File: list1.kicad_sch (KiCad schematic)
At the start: 10 parts, among them U1 8284A, U2 8259A, U22 74LS04, U3 8088, Y1 14.31818MHz

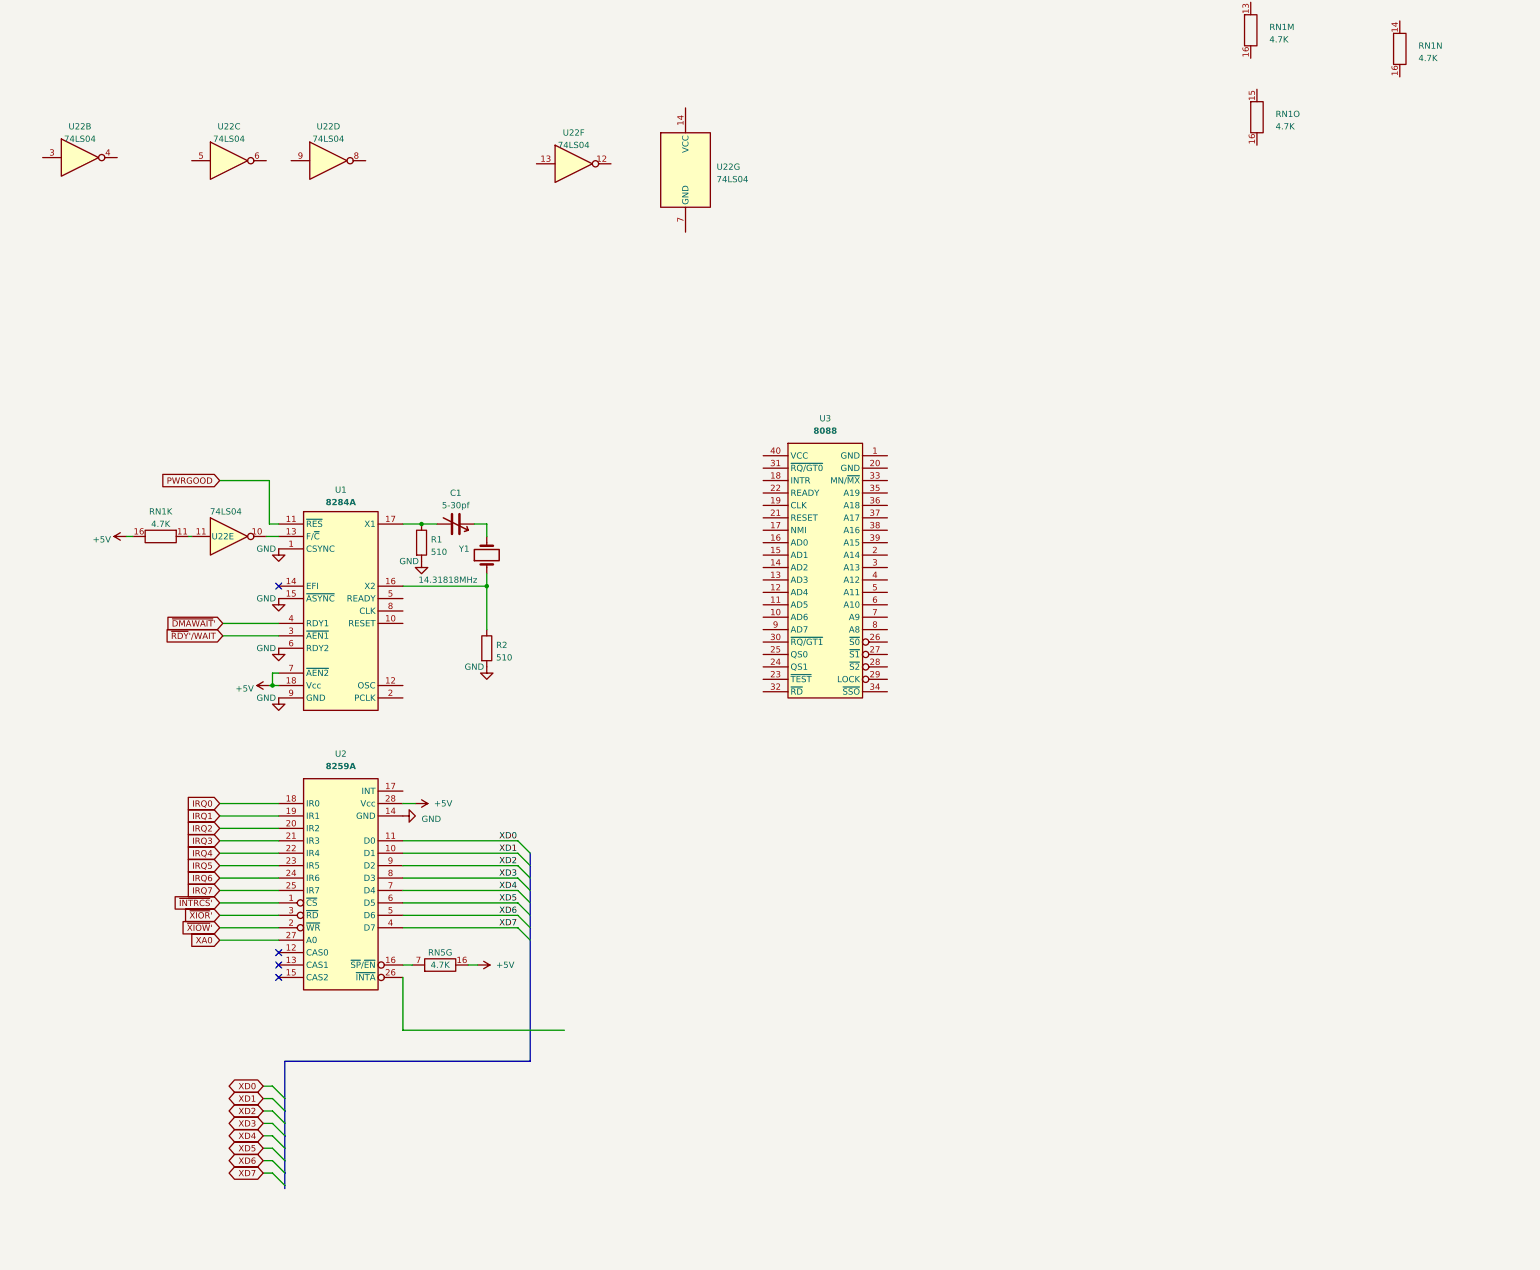
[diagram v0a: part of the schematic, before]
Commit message: Small update 18.04.2024
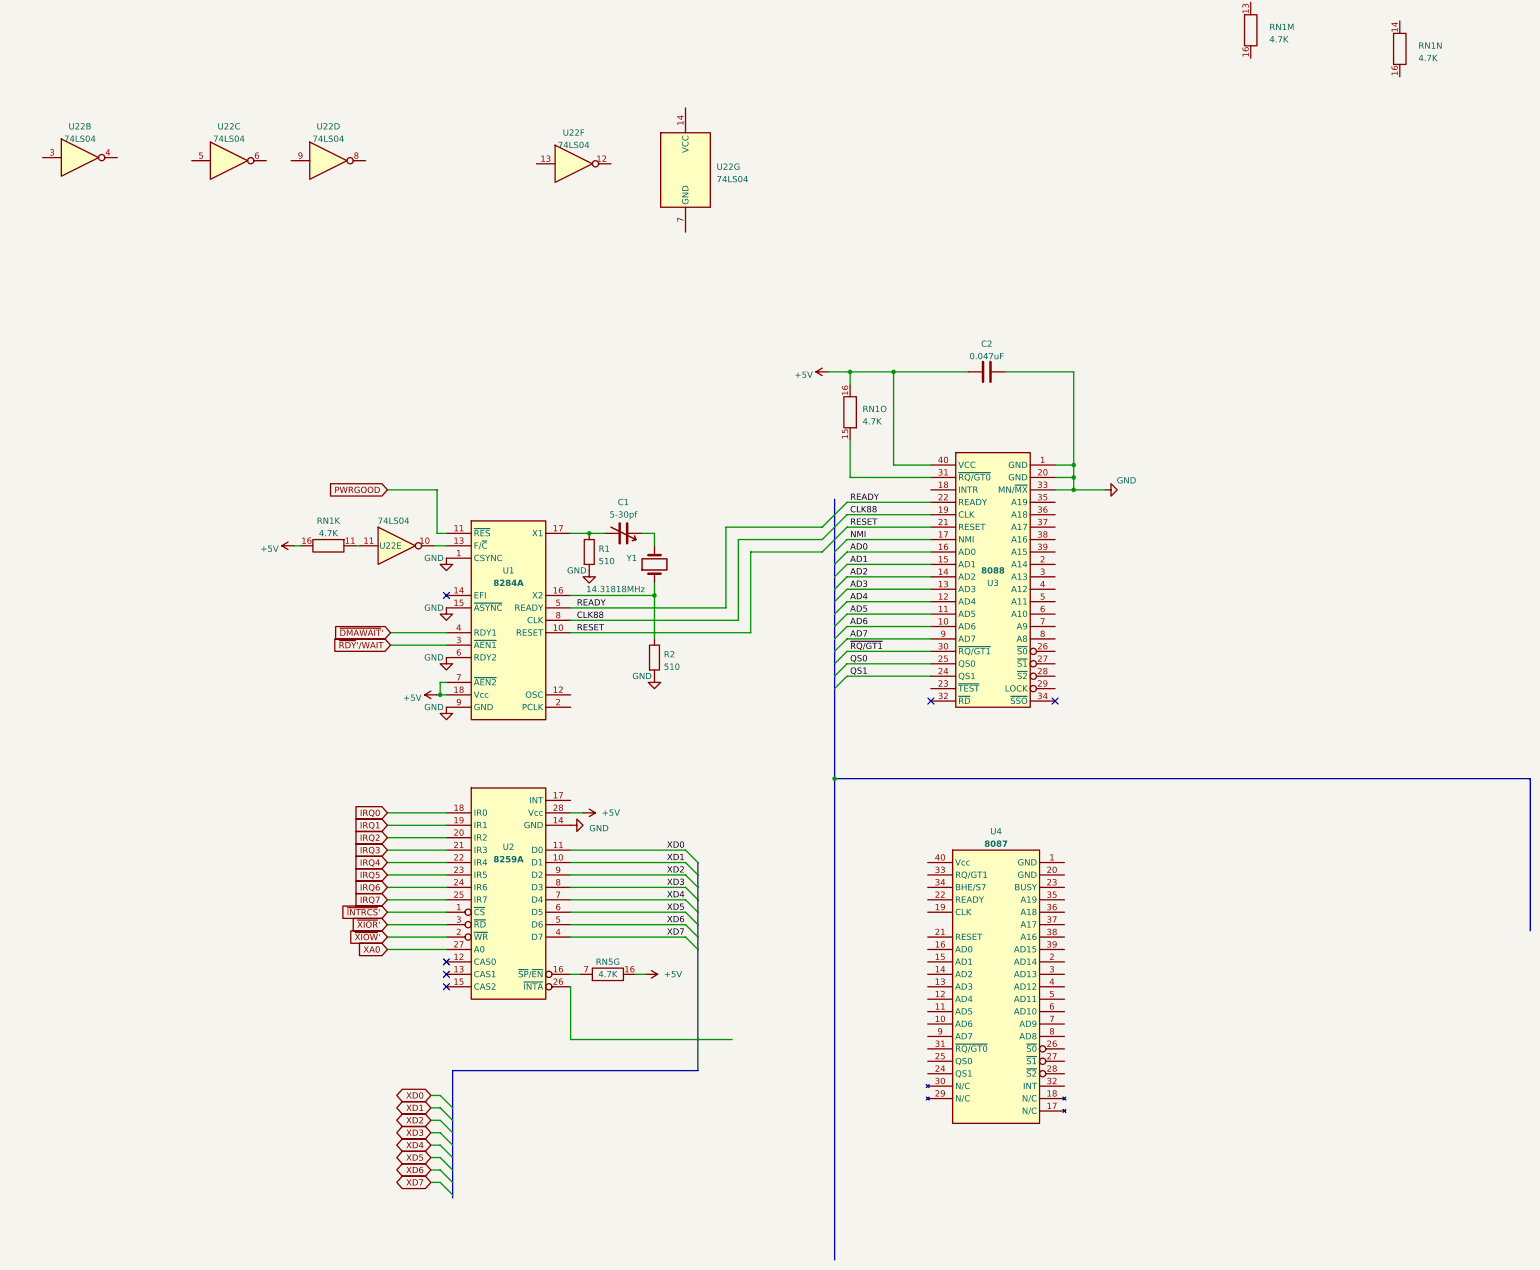
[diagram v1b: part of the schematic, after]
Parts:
- added C2: 0.047uF, symbol Device:C
- added U4: 8087, Package_DIP:DIP-40_W15.24mm_Socket_LongPads, symbol Mad5150_early:8087
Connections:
- net +5V: now also RN1.16, U3.40 (VCC), C2.1
- net GND: now also U3.1 (GND), U3.20 (GND), U3.33 (MN/~{MX}), C2.2
- net AD6: now reaches U3.10 (AD6)
- net AD5: now reaches U3.11 (AD5)
- net AD4: now reaches U3.12 (AD4)
- net AD3: now reaches U3.13 (AD3)
- net AD2: now reaches U3.14 (AD2)
- net AD1: now reaches U3.15 (AD1)
- net AD0: now reaches U3.16 (AD0)
- net NMI: now reaches U3.17 (NMI)
- net CLK88: now reaches U3.19 (CLK)
- net CLK88: now also U1.8 (CLK)
- net RESET: now reaches U3.21 (RESET)
- net RESET: now also U1.10 (RESET)
- net READY: now reaches U3.22 (READY)
- net READY: now also U1.5 (READY)
- net QS1: now reaches U3.24 (QS1)
- net QS0: now reaches U3.25 (QS0)
- net ~{RQ/GT1}: now reaches U3.30 (~{RQ/GT1})
- net at U3.31 (~{RQ/GT0}): now also RN1.15
- net AD7: now reaches U3.9 (AD7)
- no-connect marks 4 -> 6
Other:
- moved on the sheet: C1, R1, R2, RN1K, RN5G, U1, U2, U22E, U3, Y1
